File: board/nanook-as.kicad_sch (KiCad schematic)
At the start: 22 parts, among them J1 Water Flow, J2 Address, J3 USB, U1 CD4051B, U2 ESP32-C3FN4, X1 I2C-6P, Y1 40MHz

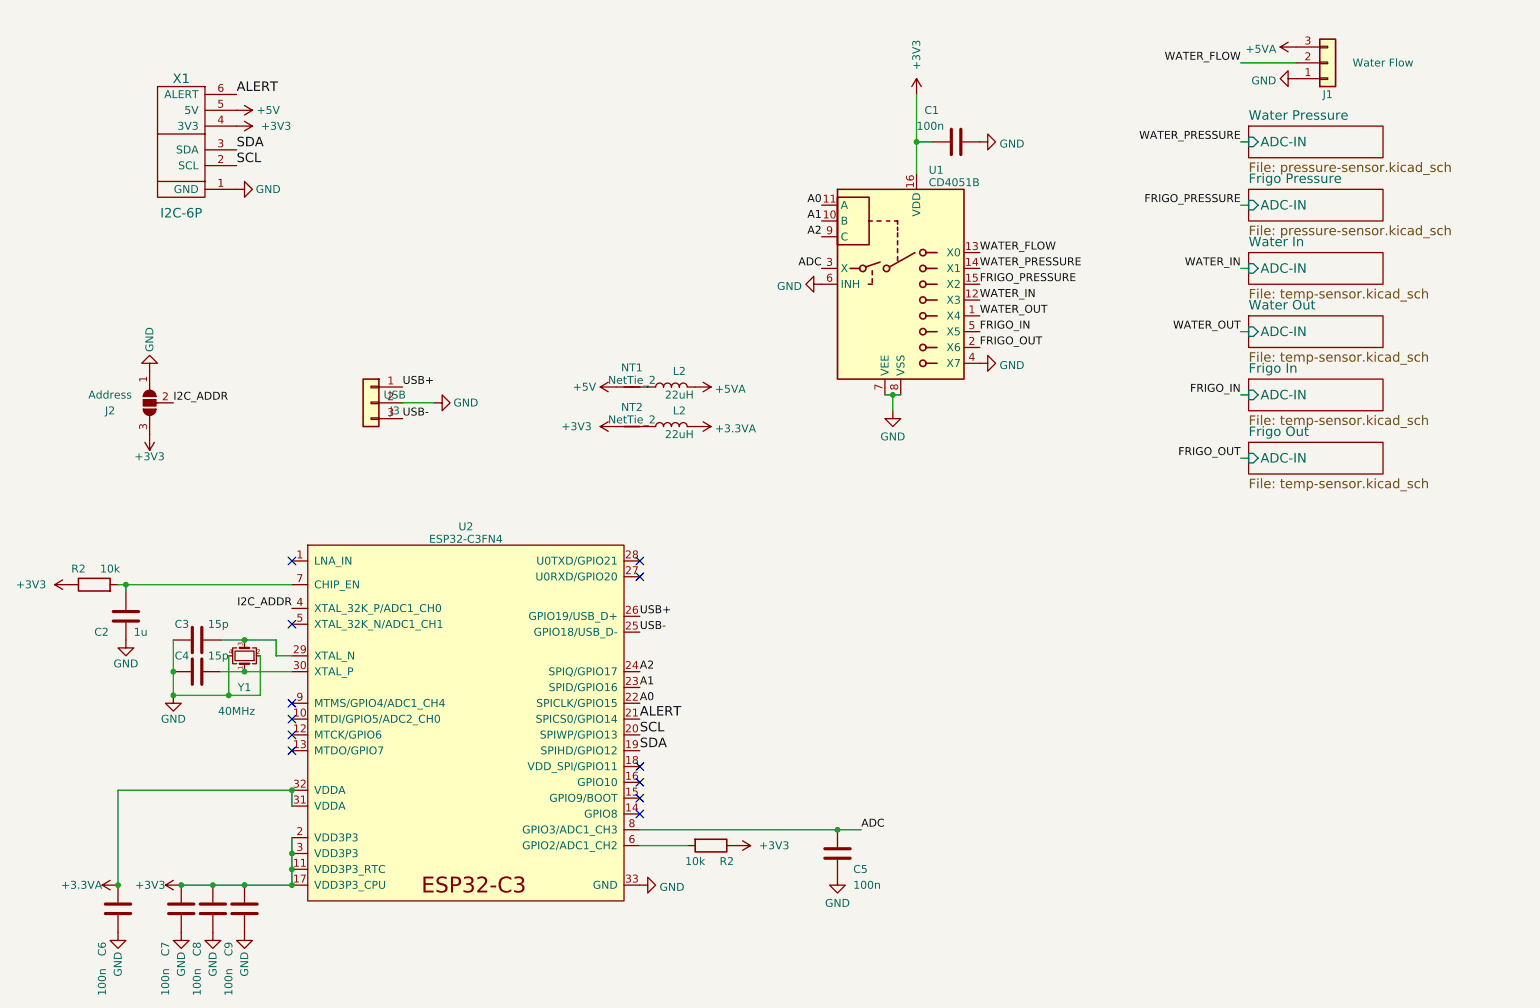
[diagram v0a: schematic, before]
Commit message: WIP
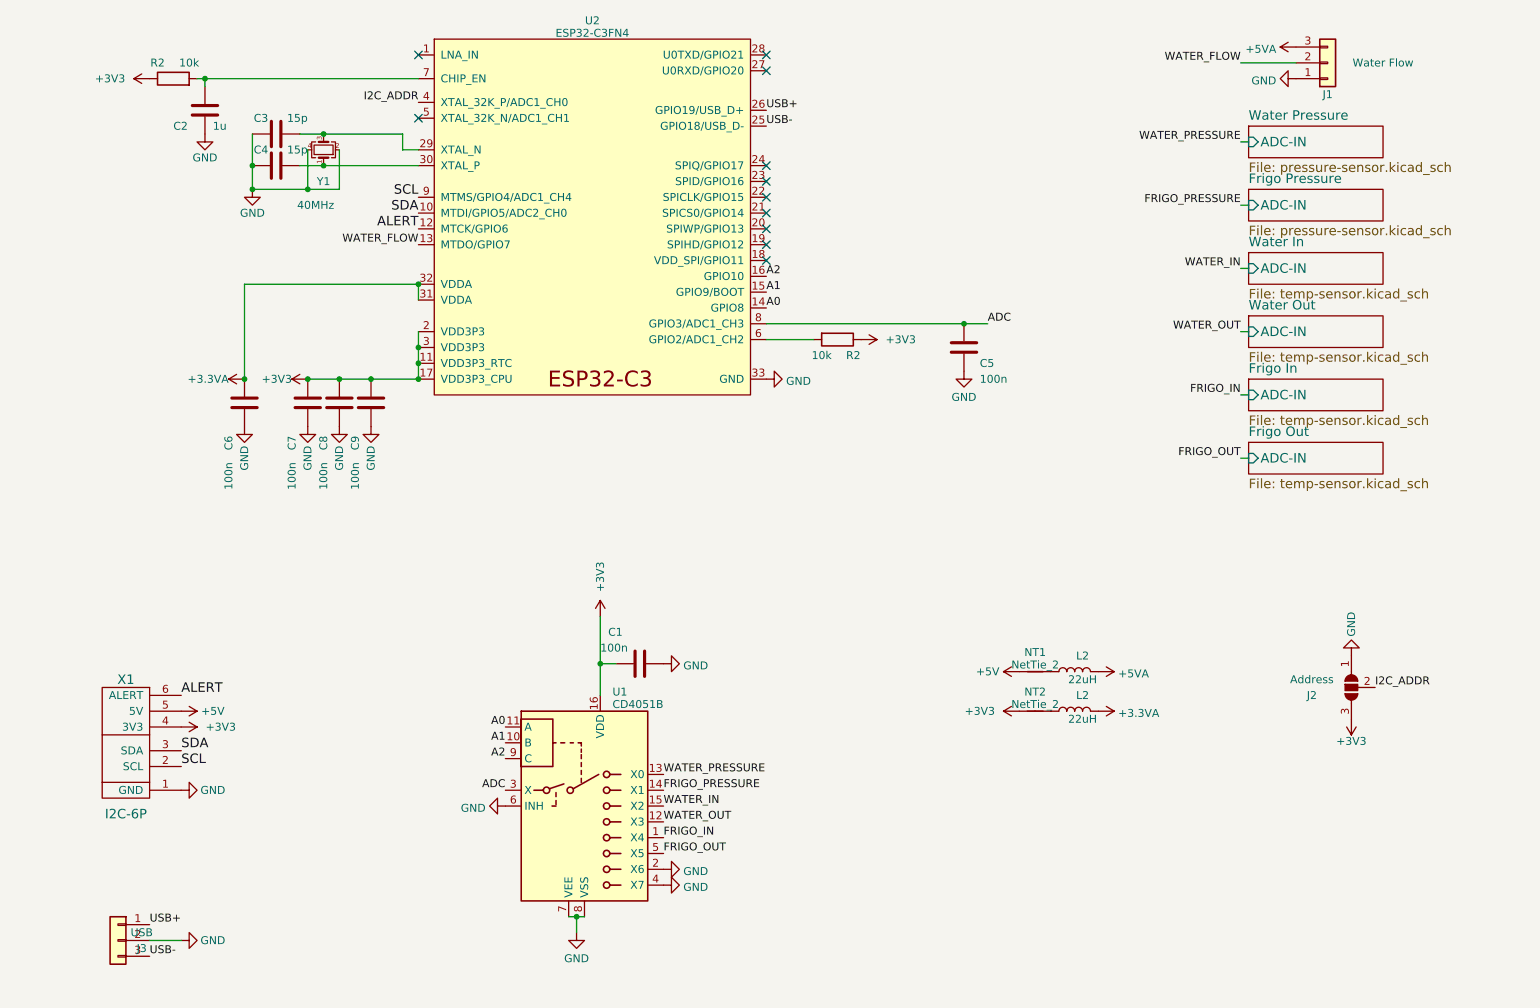
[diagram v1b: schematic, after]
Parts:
- Y1: footprint Crystal:Crystal_SMD_3225-4Pin_3.2x2.5mm_HandSoldering -> Crystal:Crystal_SMD_3225-4Pin_3.2x2.5mm
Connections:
- net A0: now also U2.14 (GPIO8); no longer U2.22 (SPICLK/GPIO15)
- net A1: now also U2.15 (GPIO9/BOOT); no longer U2.23 (SPID/GPIO16)
- net A2: now also U2.16 (GPIO10); no longer U2.24 (SPIQ/GPIO17)
- net ALERT: now also U2.12 (MTCK/GPIO6); no longer U2.21 (SPICS0/GPIO14)
- net FRIGO_IN: now also U1.1 (X4); no longer U1.5 (X5)
- net FRIGO_OUT: now also U1.5 (X5); no longer U1.2 (X6)
- net FRIGO_PRESSURE: now also U1.14 (X1); no longer U1.15 (X2)
- net GND: now also U1.2 (X6)
- net SCL: now also U2.9 (MTMS/GPIO4/ADC1_CH4); no longer U2.20 (SPIWP/GPIO13)
- net SDA: now also U2.10 (MTDI/GPIO5/ADC2_CH0); no longer U2.19 (SPIHD/GPIO12)
- net WATER_FLOW: now also U2.13 (MTDO/GPIO7); no longer U1.13 (X0)
- net WATER_IN: now also U1.15 (X2); no longer U1.12 (X3)
- net WATER_OUT: now also U1.12 (X3); no longer U1.1 (X4)
- net WATER_PRESSURE: now also U1.13 (X0); no longer U1.14 (X1)
- no-connect marks 12 -> 11
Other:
- moved on the sheet: C1, C2, C3, C4, C5, C6, C7, C8, C9, J2, J3, L2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
